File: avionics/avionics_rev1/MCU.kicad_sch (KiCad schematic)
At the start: 36 parts, among them J5 FTSH-107-01-L-DV-K, Q2 DMN2056U-7, U14 W25Q512JVFIM, U2 STM32G474RET6, Y1 16MHz / CL10pF

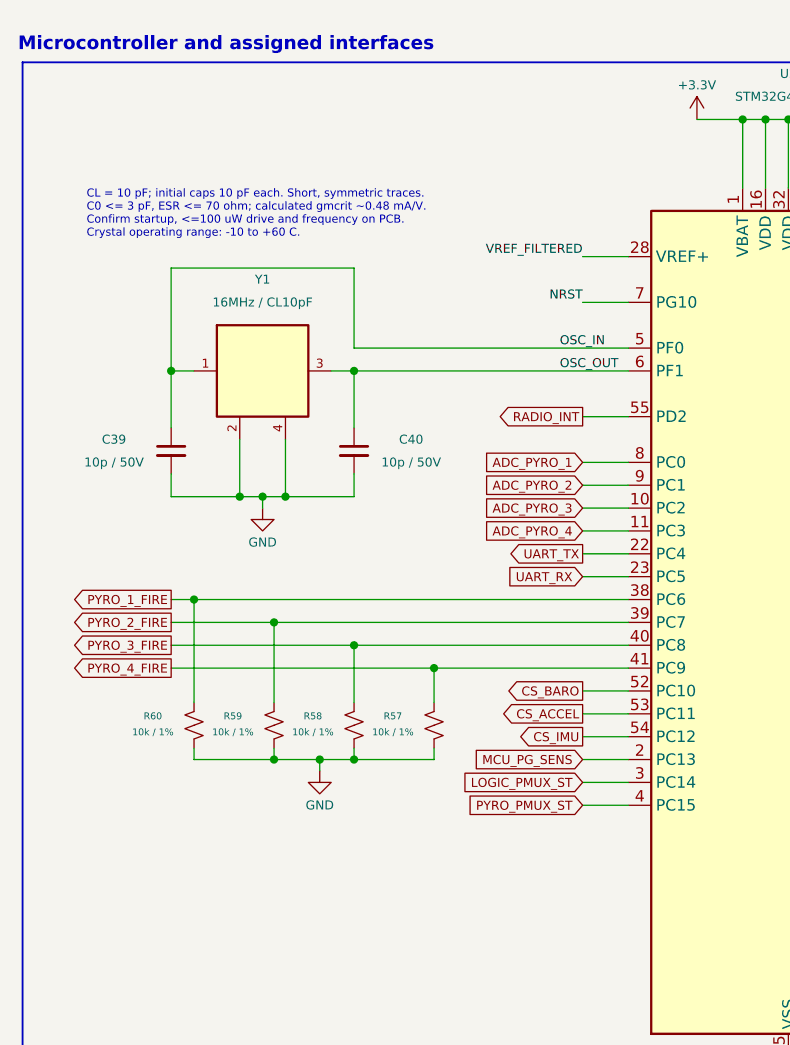
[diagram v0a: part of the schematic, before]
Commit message: saving MCU work before using codex
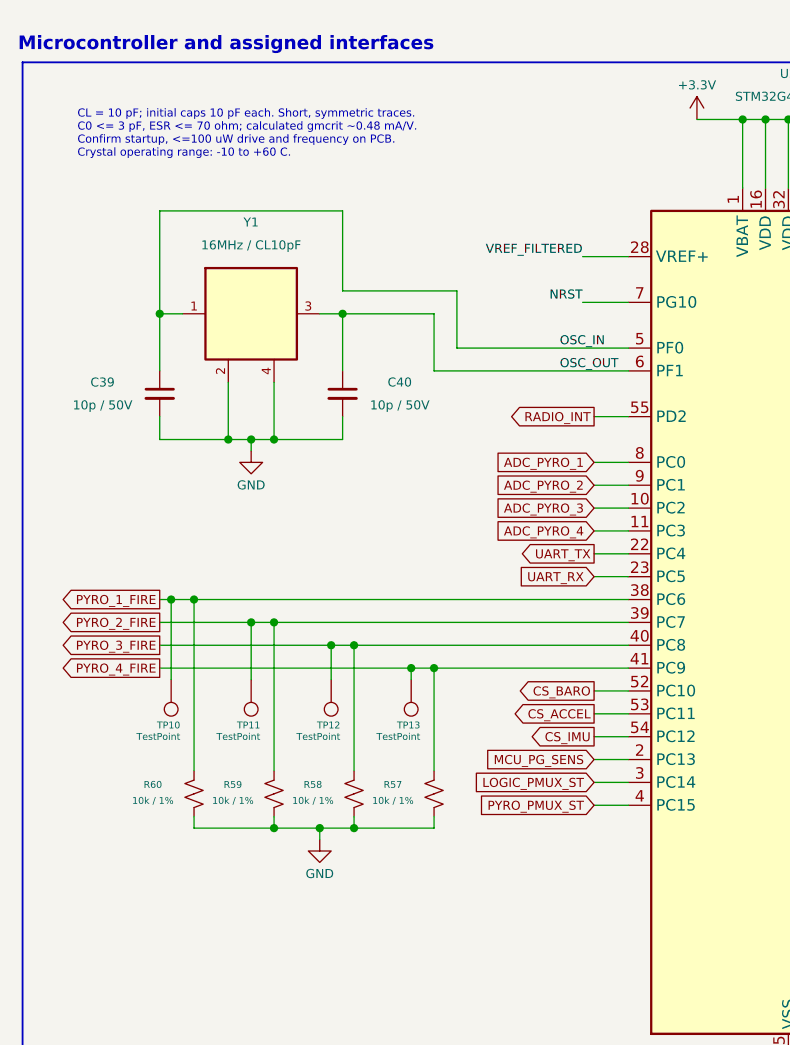
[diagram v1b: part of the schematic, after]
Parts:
- added TP10, TP11, TP12, TP13: TestPoint, symbol Connector:TestPoint
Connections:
- net PYRO_1_FIRE: now also TP10.1
- net PYRO_2_FIRE: now also TP11.1
- net PYRO_3_FIRE: now also TP12.1
- net PYRO_4_FIRE: now also TP13.1
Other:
- moved on the sheet: C39, C40, R57, R58, R59, R60, Y1
